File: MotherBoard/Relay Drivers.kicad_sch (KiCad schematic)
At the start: 28 parts, among them Q701 Q_NPN_BEC, Q702 Q_NPN_BEC, Q703 Q_NPN_BEC, Q704 Q_NMOS_GDS, Q705 Q_NMOS_GDS, Q706 Q_NMOS_GDS, Q707 Q_NPN_BEC, Q708 Q_NMOS_GDS

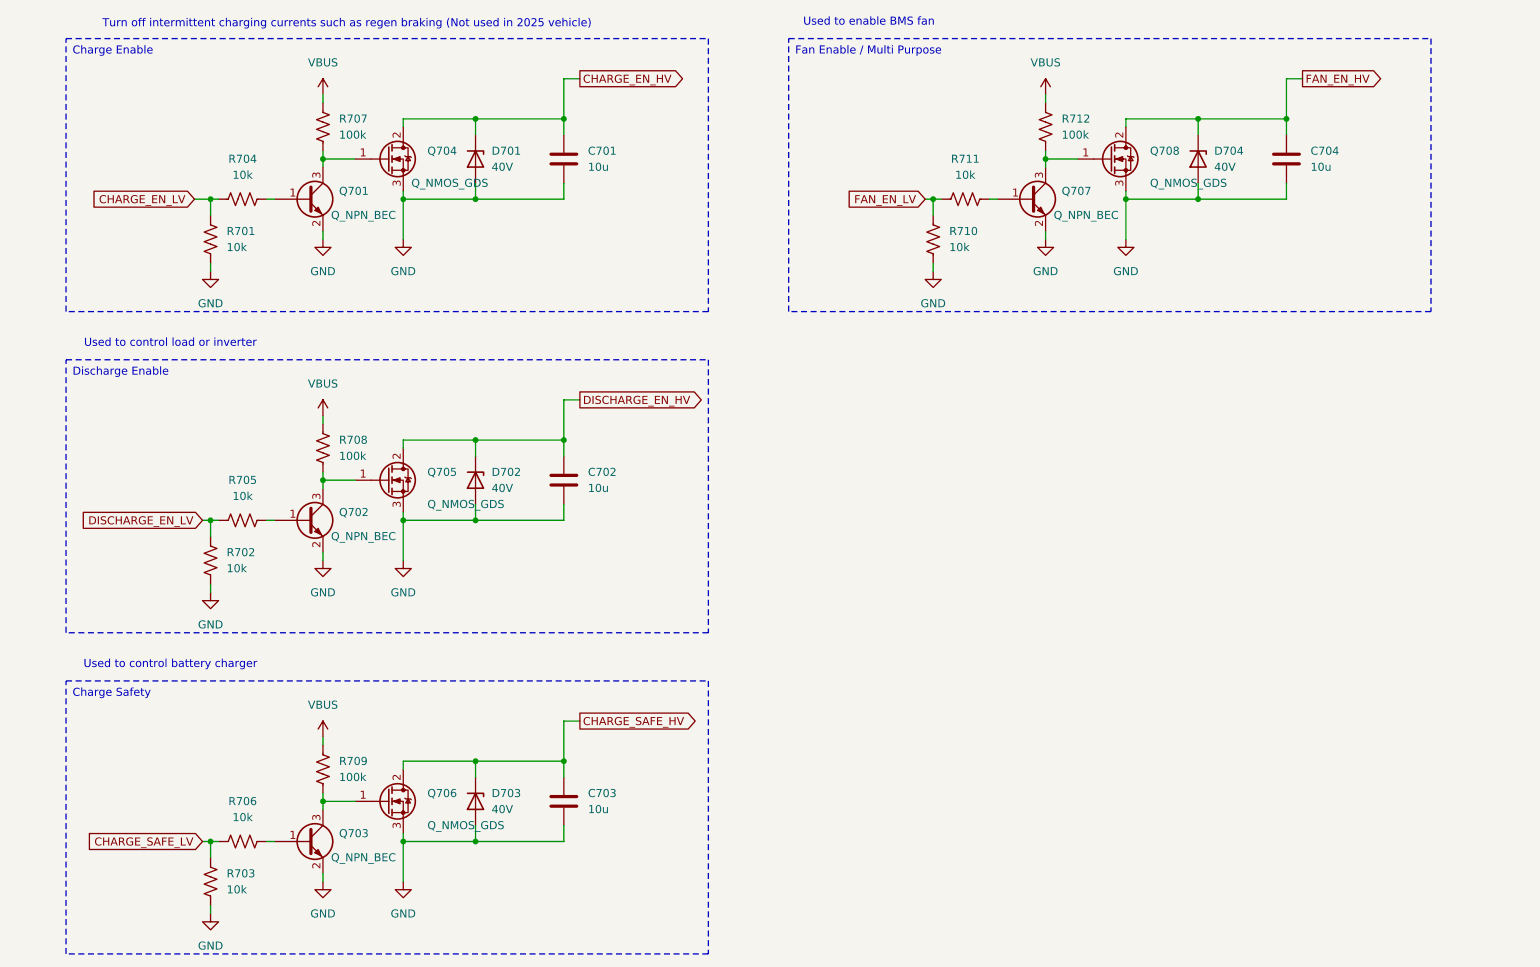
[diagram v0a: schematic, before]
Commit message: Daughterboard 100% Complete + Edited Motherboard BOM
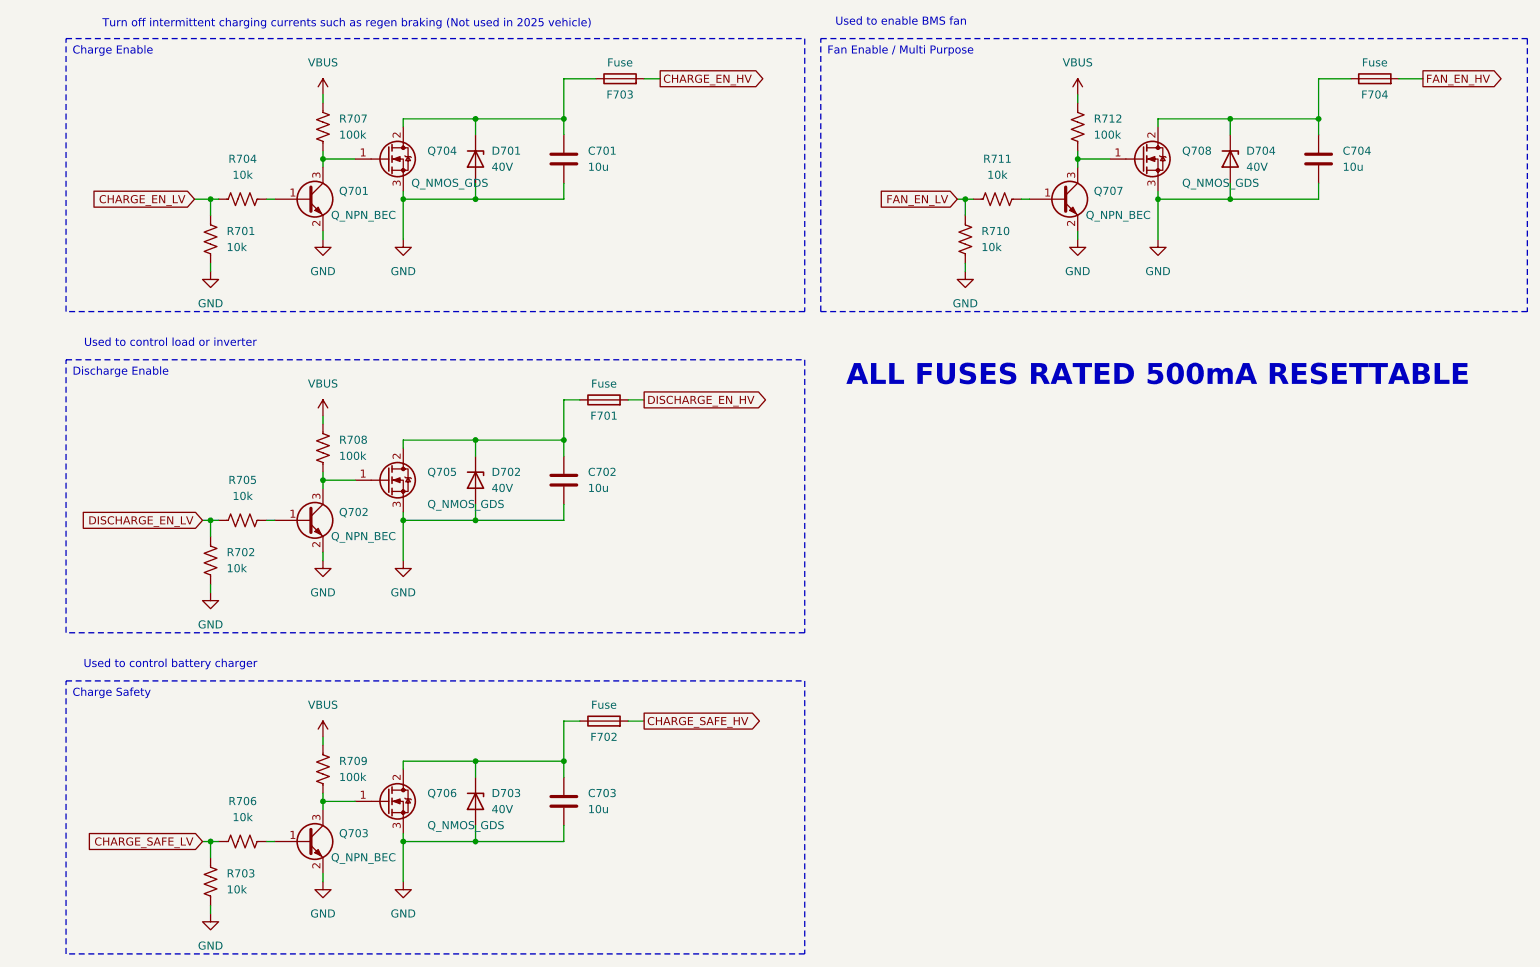
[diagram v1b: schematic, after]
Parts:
- added F701, F702, F703, F704: Fuse, Fuse:Fuse_1812_4532Metric, symbol Device:Fuse
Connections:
- net CHARGE_EN_HV: now also F703.2; no longer C701.1, D701.1 (K), Q704.2 (D)
- net CHARGE_SAFE_HV: now also F702.2; no longer C703.1, D703.1 (K), Q706.2 (D)
- net DISCHARGE_EN_HV: now also F701.2; no longer C702.1, D702.1 (K), Q705.2 (D)
- net FAN_EN_HV: now also F704.2; no longer C704.1, D704.1 (K), Q708.2 (D)
- new net: C704.1, D704.1 (K), F704.1, Q708.2 (D)
- new net: C702.1, D702.1 (K), F701.1, Q705.2 (D)
- new net: C703.1, D703.1 (K), F702.1, Q706.2 (D)
- new net: C701.1, D701.1 (K), F703.1, Q704.2 (D)
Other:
- note added: "ALL FUSES RATED 500mA RESETTABLE"
- moved on the sheet: C704, D704, Q707, Q708, R710, R711, R712

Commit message: Both boards complete
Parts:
- C701, C702, C703, C704: JLCPCB Part # (none) -> C13585
- D701, D702, D703, D704: JLCPCB Part # (none) -> C19077418
- F701, F702, F703, F704: JLCPCB Part # (none) -> C12559
- Q701, Q702, Q703, Q707: JLCPCB Part # (none) -> C7420353
- Q704, Q705, Q706, Q708: JLCPCB Part # (none) -> C2613
- R701, R702, R703, R704, R705, R706, R710, R711: JLCPCB Part # (none) -> C2930027; Manufacturer_Part_Number 0402WGF1001TCE -> FRC0603J103TS
- R707, R708, R709, R712: JLCPCB Part # (none) -> C25741
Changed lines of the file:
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@@
 			)
 		)
-		(property "JLC" ""
+		(property "JLCPCB Part #" "C13585"
 			(at 223.52 44.45 0)
 			(effects
@@
 			)
 		)
-		(property "JLC" ""
+		(property "JLCPCB Part #" "C25741"
 			(at 185.42 39.37 0)
 			(effects
@@
 			)
 		)
+		(property "JLCPCB Part #" "C12559"
+			(at 110.49 82.55 0)
+			(effects
+				(font
+					(size 1.27 1.27)
+				)
+				(hide yes)
+			)
+		)
 		(pin "2"
 		)
@@
 			)
 		)
-		(property "Manufacturer_Part_Number" "0402WGF1001TCE"
+		(property "Manufacturer_Part_Number" "FRC0603J103TS"
 			(at 48.26 57.15 0)
 			(effects
@@
 			)
 		)
-		(property "JLC" ""
+		(property "JLCPCB Part #" "C2930027"
 			(at 48.26 57.15 0)
 			(effects
@@
 			)
 		)
+		(property "JLCPCB Part #" "C12559"
+			(at 110.49 133.35 0)
+			(effects
+				(font
+					(size 1.27 1.27)
+				)
+				(hide yes)
+			)
+		)
 		(pin "2"
 		)
@@
 			)
 		)
-		(property "Manufacturer_Part_Number" "0402WGF1001TCE"
+		(property "Manufacturer_Part_Number" "FRC0603J103TS"
 			(at 53.34 152.4 0)
 			(effects
@@
 			)
 		)
-		(property "JLC" ""
+		(property "JLCPCB Part #" "C2930027"
 			(at 53.34 152.4 0)
 			(effects
@@
 			)
 		)
-		(property "JLC" ""
+		(property "JLCPCB Part #" "C2613"
 			(at 195.58 44.45 0)
 			(effects
@@
 			)
 		)
-		(property "Manufacturer_Part_Number" "0402WGF1001TCE"
+		(property "Manufacturer_Part_Number" "FRC0603J103TS"
 			(at 172.72 50.8 0)
 			(effects
@@
 			)
 		)
-		(property "JLC" ""
+		(property "JLCPCB Part #" "C2930027"
 			(at 172.72 50.8 0)
 			(effects
@@
 			)
 		)
-		(property "JLC" ""
+		(property "JLCPCB Part #" "C7420353"
 			(at 63.5 152.4 0)
 			(effects
@@
 			)
 		)
-		(property "Manufacturer_Part_Number" "0402WGF1001TCE"
+		(property "Manufacturer_Part_Number" "FRC0603J103TS"
 			(at 48.26 158.75 0)
 			(effects
@@
 			)
 		)
-		(property "JLC" ""
+		(property "JLCPCB Part #" "C2930027"
 			(at 48.26 158.75 0)
 			(effects
@@
 			)
 		)
-		(property "JLC" ""
+		(property "JLCPCB Part #" "C13585"
 			(at 104.14 44.45 0)
 			(effects
@@
 			)
 		)
-		(property "JLC" ""
+		(property "JLCPCB Part #" "C19077418"
 			(at 209.55 44.45 0)
 			(effects
@@
 			)
 		)
+		(property "JLCPCB Part #" "C12559"
+			(at 113.03 31.75 0)
+			(effects
+				(font
+					(size 1.27 1.27)
+				)
+				(hide yes)
+			)
+		)
 		(pin "2"
 		)
@@
 			)
 		)
-		(property "JLC" ""
+		(property "JLCPCB Part #" "C25741"
 			(at 66.04 39.37 0)
 			(effects
@@
 			)
 		)
-		(property "JLC" ""
+		(property "JLCPCB Part #" "C19077418"
 			(at 90.17 95.25 0)
 			(effects
@@
 			)
 		)
-		(property "JLC" ""
+		(property "JLCPCB Part #" "C2613"
 			(at 76.2 146.05 0)
 			(effects
@@
 			)
 		)
-		(property "JLC" ""
+		(property "JLCPCB Part #" "C7420353"
 			(at 63.5 50.8 0)
 			(effects
@@
 			)
 		)
-		(property "Manufacturer_Part_Number" "0402WGF1001TCE"
+		(property "Manufacturer_Part_Number" "FRC0603J103TS"
 			(at 167.64 57.15 0)
 			(effects
@@
 			)
 		)
-		(property "JLC" ""
+		(property "JLCPCB Part #" "C2930027"
 			(at 167.64 57.15 0)
 			(effects
@@
 			)
 		)
-		(property "JLC" ""
+		(property "JLCPCB Part #" "C25741"
 			(at 66.04 90.17 0)
 			(effects
@@
 			)
 		)
-		(property "Manufacturer_Part_Number" "0402WGF1001TCE"
+		(property "Manufacturer_Part_Number" "FRC0603J103TS"
 			(at 53.34 50.8 0)
 			(effects
@@
 			)
 		)
-		(property "JLC" ""
+		(property "JLCPCB Part #" "C2930027"
 			(at 53.34 50.8 0)
 			(effects
@@
 			)
 		)
-		(property "Manufacturer_Part_Number" "0402WGF1001TCE"
+		(property "Manufacturer_Part_Number" "FRC0603J103TS"
 			(at 53.34 101.6 0)
 			(effects
@@
 			)
 		)
-		(property "JLC" ""
+		(property "JLCPCB Part #" "C2930027"
 			(at 53.34 101.6 0)
 			(effects
@@
 			)
 		)
-		(property "Manufacturer_Part_Number" "0402WGF1001TCE"
+		(property "Manufacturer_Part_Number" "FRC0603J103TS"
 			(at 48.26 107.95 0)
 			(effects
@@
 			)
 		)
-		(property "JLC" ""
+		(property "JLCPCB Part #" "C2930027"
 			(at 48.26 107.95 0)
 			(effects
@@
 			)
 		)
+		(property "JLCPCB Part #" "C12559"
+			(at 232.41 31.75 0)
+			(effects
+				(font
+					(size 1.27 1.27)
+				)
+				(hide yes)
+			)
+		)
 		(pin "2"
 		)
@@
 			)
 		)
-		(property "JLC" ""
+		(property "JLCPCB Part #" "C25741"
 			(at 66.04 140.97 0)
 			(effects
@@
 			)
 		)
-		(property "JLC" ""
+		(property "JLCPCB Part #" "C13585"
 			(at 104.14 146.05 0)
 			(effects
@@
 			)
 		)
-		(property "JLC" ""
+		(property "JLCPCB Part #" "C2613"
 			(at 76.2 44.45 0)
 			(effects
@@
 			)
 		)
-		(property "JLC" ""
+		(property "JLCPCB Part #" "C19077418"
 			(at 90.17 146.05 0)
 			(effects
@@
 			)
 		)
-		(property "JLC" ""
+		(property "JLCPCB Part #" "C7420353"
 			(at 182.88 50.8 0)
 			(effects
@@
 			)
 		)
-		(property "JLC" ""
+		(property "JLCPCB Part #" "C13585"
 			(at 104.14 95.25 0)
 			(effects
@@
 			)
 		)
-		(property "JLC" ""
+		(property "JLCPCB Part #" "C2613"
 			(at 76.2 95.25 0)
 			(effects
@@
 			)
 		)
-		(property "JLC" ""
+		(property "JLCPCB Part #" "C19077418"
 			(at 90.17 44.45 0)
 			(effects
@@
 			)
 		)
-		(property "JLC" ""
+		(property "JLCPCB Part #" "C7420353"
 			(at 63.5 101.6 0)
 			(effects
